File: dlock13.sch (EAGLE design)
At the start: 18 parts, among them IC2 7805T, Q1 IRLZ44Z, Q2 IRLZ44Z

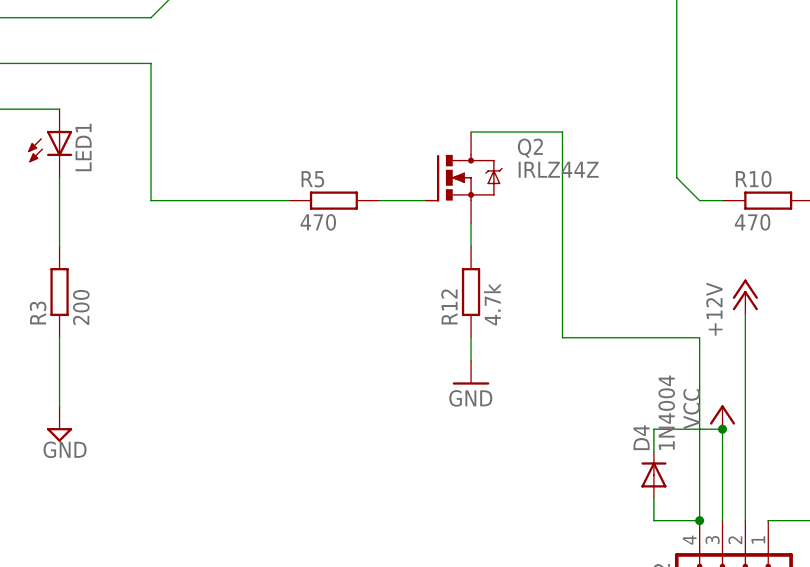
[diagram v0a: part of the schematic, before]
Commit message: Updated.
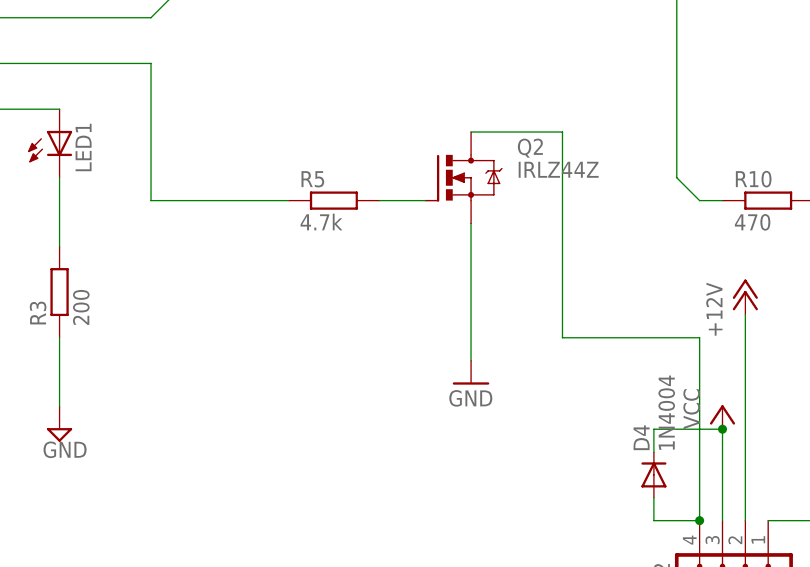
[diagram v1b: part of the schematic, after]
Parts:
- removed R12: 4.7k, rcl:R-EU_0207/10
- R5: value 470 -> 4.7k
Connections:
- removed net N$6: Q2.S, R12.2
- net GND: now also Q2.S; no longer R12.1
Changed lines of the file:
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@@
 <part name="GND4" library="supply1" deviceset="GND" device=""/>
 <part name="Q2" library="transistor-power" deviceset="IRLZ44Z" device=""/>
-<part name="R5" library="resistor" deviceset="R-EU_" device="0204/7" value="470"/>
-<part name="R12" library="rcl" deviceset="R-EU_" device="0207/10" value="4.7k"/>
+<part name="R5" library="resistor" deviceset="R-EU_" device="0204/7" value="4.7k"/>
 <part name="GND2" library="supply1" deviceset="GND" device=""/>
 <part name="P+3" library="supply1" deviceset="VCC" device=""/>
@@
 <instance part="Q2" gate="G$1" x="68.58" y="50.8"/>
 <instance part="R5" gate="G$1" x="55.88" y="48.26"/>
-<instance part="R12" gate="G$1" x="71.12" y="38.1" rot="R90"/>
 <instance part="GND2" gate="1" x="71.12" y="27.94"/>
 <instance part="P+3" gate="VCC" x="99.06" y="25.4"/>
@@
 <segment>
 <pinref part="GND2" gate="1" pin="GND"/>
-<pinref part="R12" gate="G$1" pin="1"/>
-<wire x1="71.12" y1="30.48" x2="71.12" y2="33.02" width="0.1524" layer="91"/>
+<pinref part="Q2" gate="G$1" pin="S"/>
+<wire x1="71.12" y1="30.48" x2="71.12" y2="45.72" width="0.1524" layer="91"/>
 </segment>
 <segment>
@@
 </segment>
 </net>
-<net name="N$6" class="0">
-<segment>
-<pinref part="R12" gate="G$1" pin="2"/>
-<pinref part="Q2" gate="G$1" pin="S"/>
-<wire x1="71.12" y1="43.18" x2="71.12" y2="45.72" width="0.1524" layer="91"/>
-</segment>
-</net>
